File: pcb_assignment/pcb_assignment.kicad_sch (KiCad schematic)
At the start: 4 parts, among them SW1 SW_Push

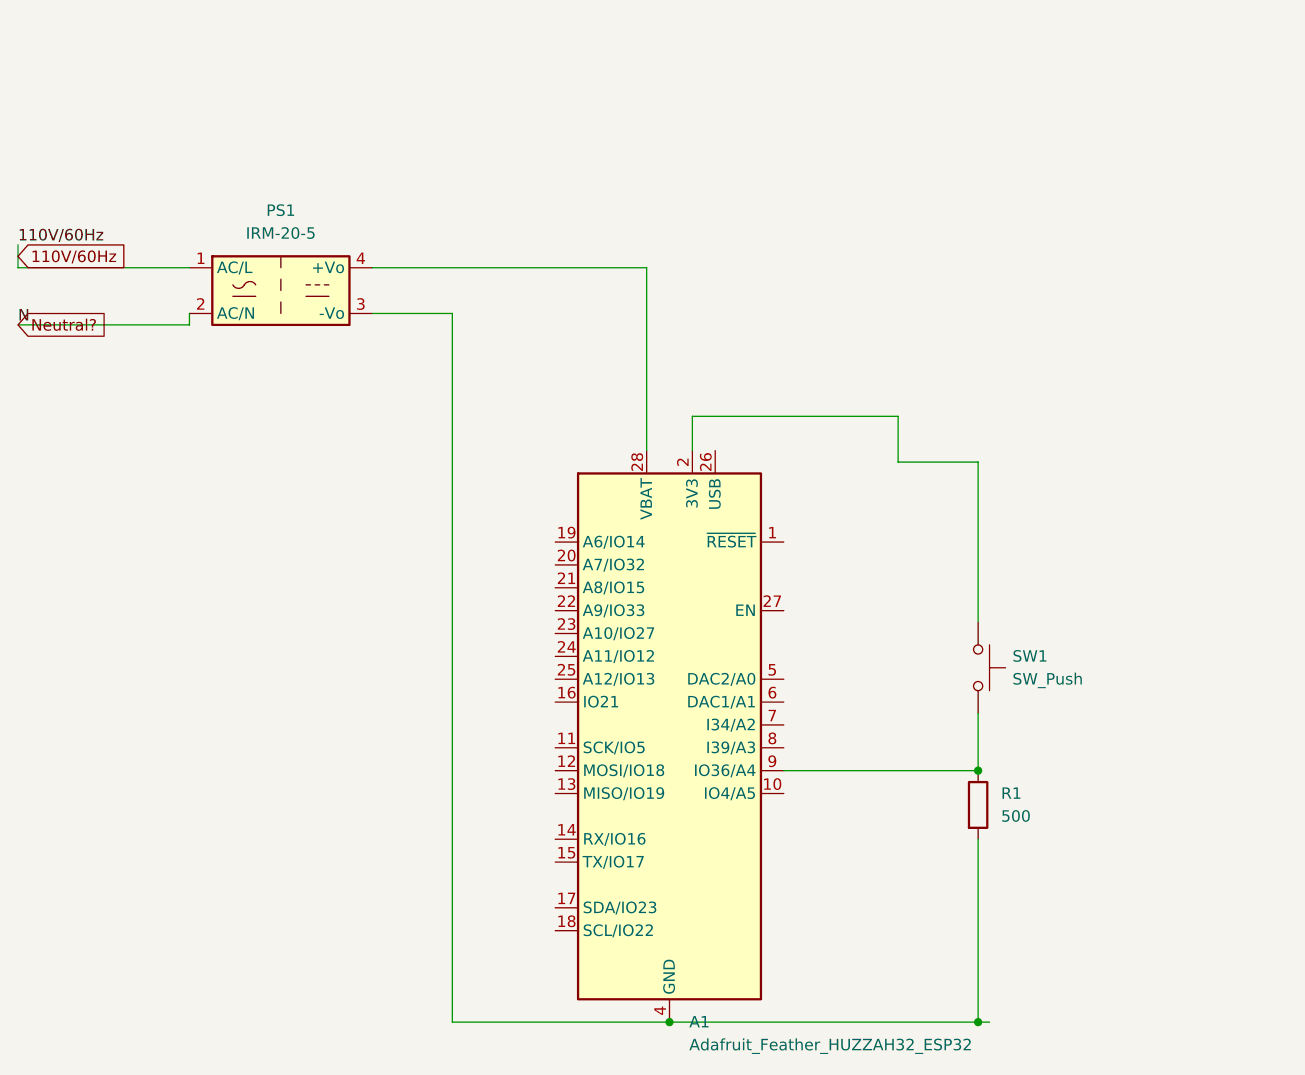
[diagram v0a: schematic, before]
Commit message: all bueno
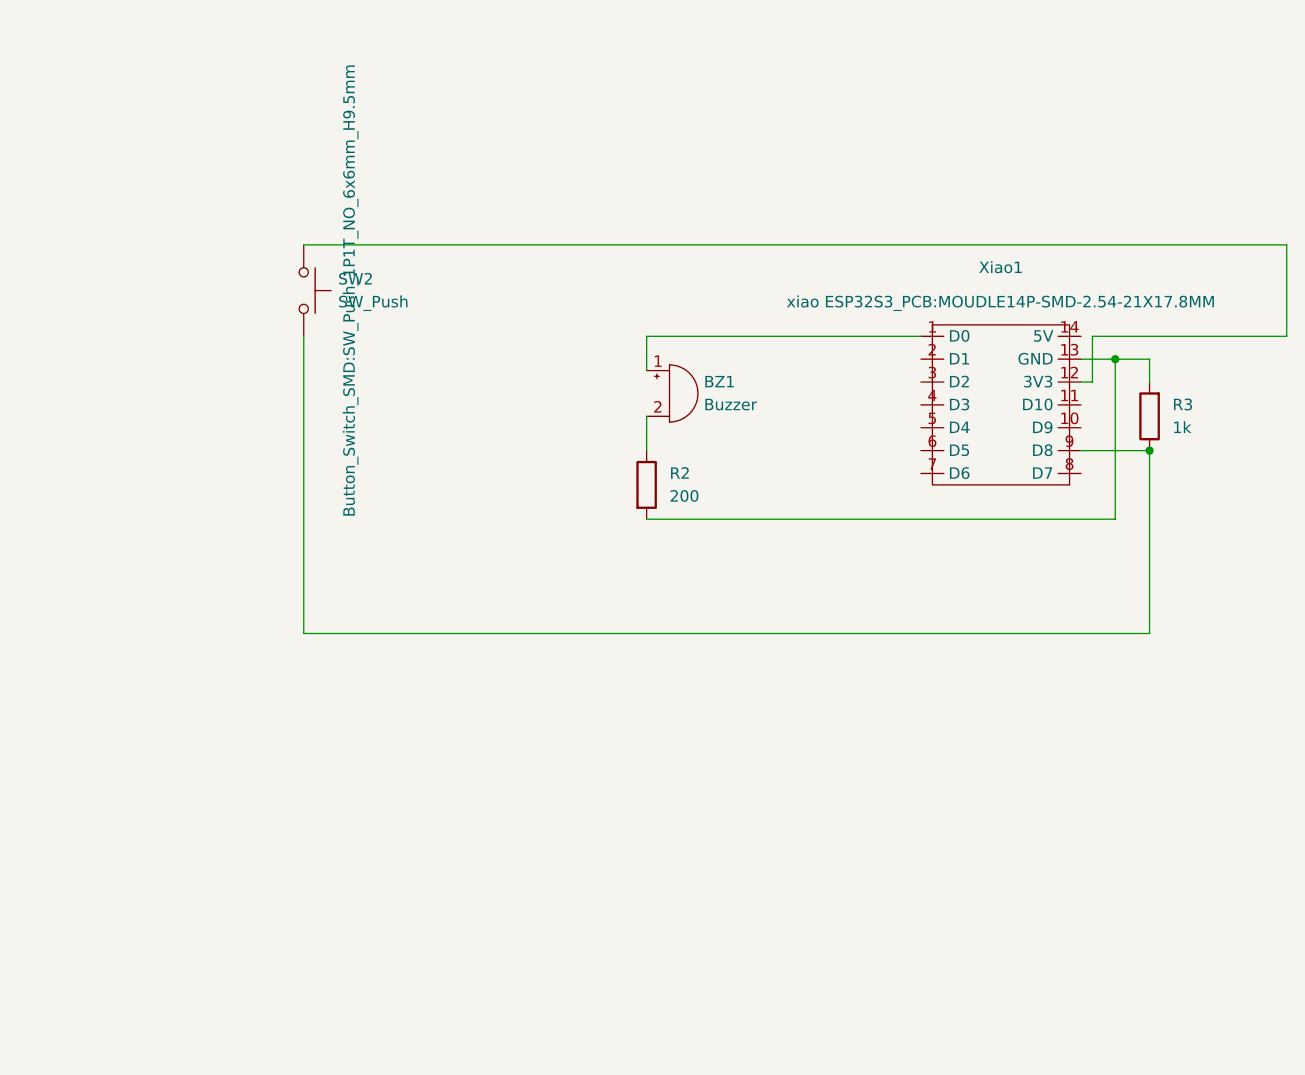
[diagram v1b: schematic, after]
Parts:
- removed A1: Adafruit_Feather_HUZZAH32_ESP32, Module:Adafruit_Feather, symbol MCU_Module:Adafruit_Feather_HUZZAH32_ESP32
- removed PS1: IRM-20-5, Converter_ACDC:Converter_ACDC_MeanWell_IRM-20-xx_THT, symbol Converter_ACDC:IRM-20-5
- removed R1: 500, symbol Device:R
- removed SW1: SW_Push, symbol Switch:SW_Push
- added BZ1: Buzzer, Buzzer_Beeper:Buzzer_15x7.5RM7.6, symbol Device:Buzzer
- added R2: 200, Resistor_THT:R_Axial_DIN0207_L6.3mm_D2.5mm_P7.62mm_Horizontal, symbol Device:R
- added R3: 1k, Resistor_THT:R_Axial_DIN0207_L6.3mm_D2.5mm_P15.24mm_Horizontal, symbol Device:R
- added SW2: SW_Push, Button_Switch_SMD:SW_Push_1P1T_NO_6x6mm_H9.5mm, symbol Switch:SW_Push
- added Xiao1: ~, xiao ESP32S3_PCB:MOUDLE14P-SMD-2.54-21X17.8MM, symbol 196ece:xiaos3sense
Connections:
- new net: BZ1.1 (+), Xiao1.1 (D0)
- new net: BZ1.2 (-), R2.1
- new net: SW2.1, Xiao1.12 (3V3)
- new net: R3.1, SW2.2, Xiao1.9 (D8)
- new net: R2.2, R3.2, Xiao1.13 (GND)
